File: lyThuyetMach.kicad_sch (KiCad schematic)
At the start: 13 parts, among them J1 USB_C_Receptacle_PowerOnly_6P, J2 Voltage_Booster, J3 TIP223, J4 Out_LED, J5 Clap_Detect, SW1 SW_SPDT, SW2 SW_SPDT, U1 74HC86

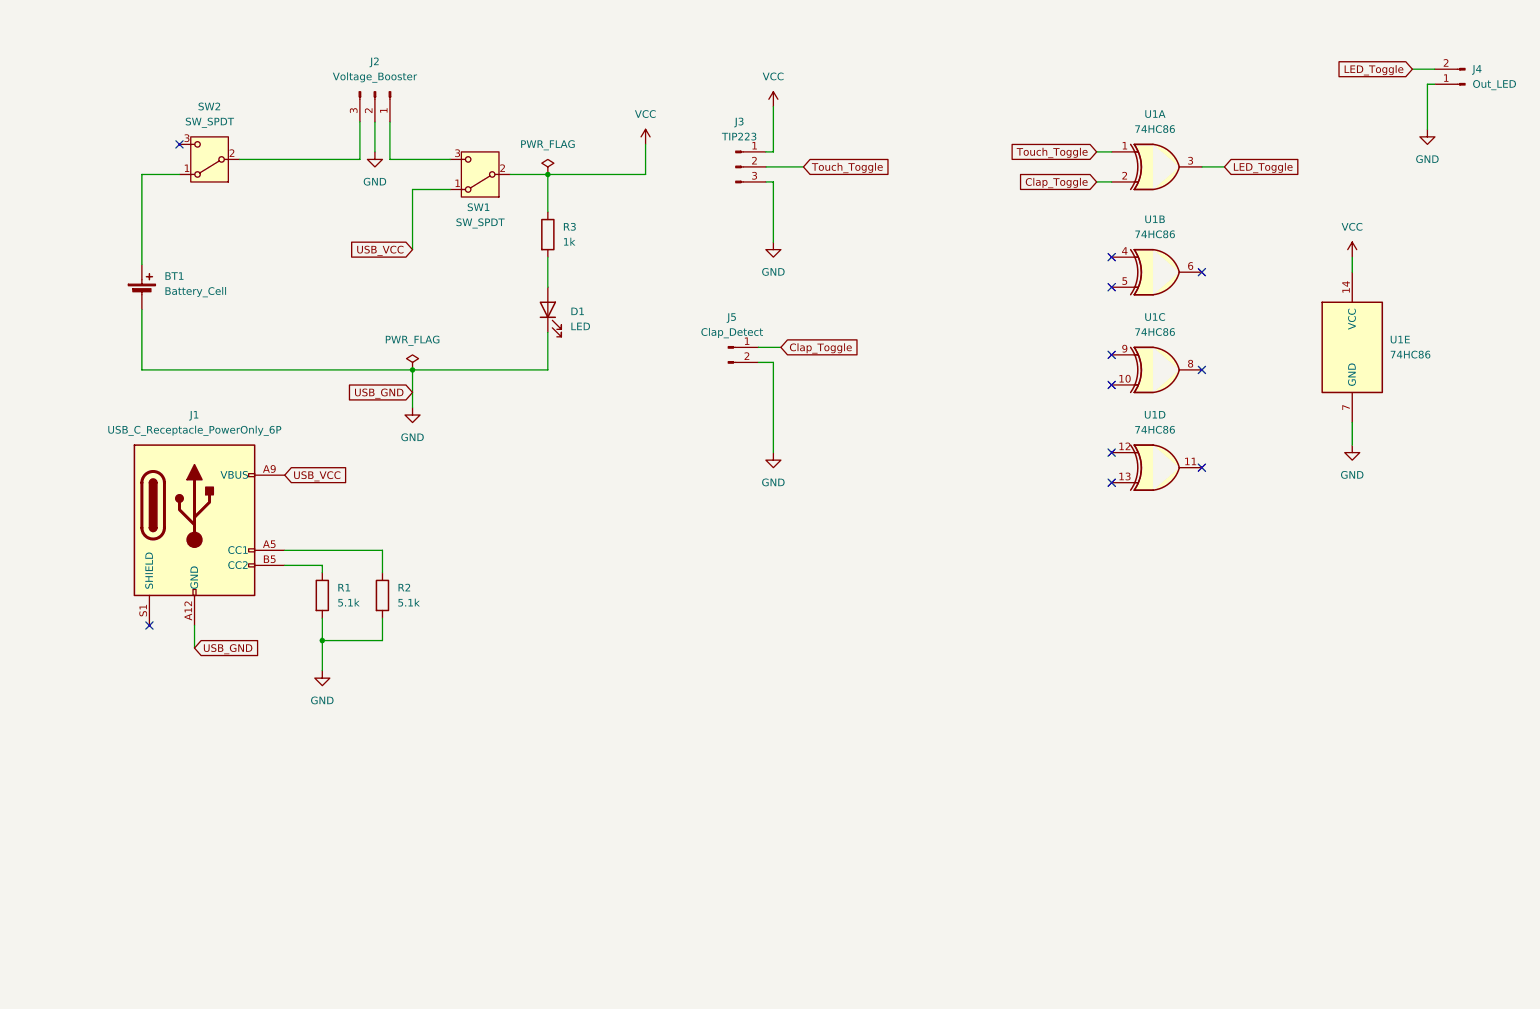
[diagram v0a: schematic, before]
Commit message: Add files via upload
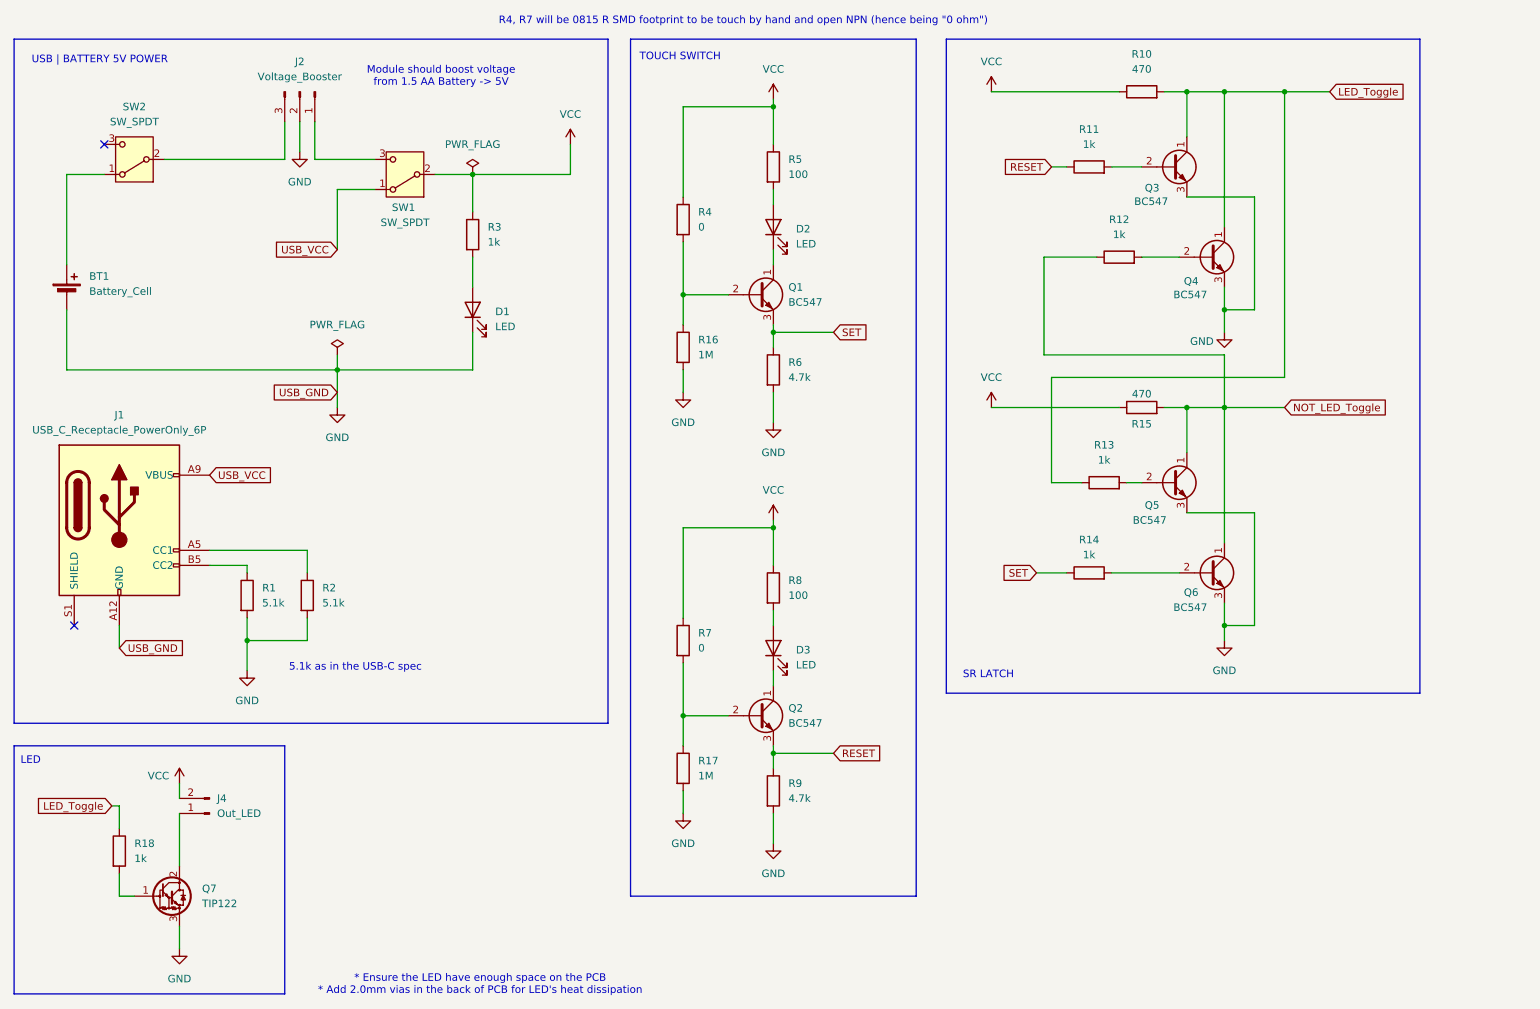
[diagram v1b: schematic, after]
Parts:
- removed J3: TIP223, Connector_PinHeader_2.54mm:PinHeader_1x03_P2.54mm_Vertical, symbol Connector:Conn_01x03_Pin
- removed J5: Clap_Detect, Connector_PinHeader_2.54mm:PinHeader_1x02_P2.54mm_Vertical, symbol Connector:Conn_01x02_Pin
- removed U1: 74HC86, Package_DIP:DIP-14_W7.62mm_Socket_LongPads, symbol 74xx:74HC86
- added D2, D3: LED, LED_THT:LED_D5.0mm_FlatTop, symbol Device:LED
- added Q1, Q2, Q3, Q4, Q5, Q6: BC547, Package_TO_SOT_THT:TO-92_Inline, symbol Transistor_BJT:BC547
- added Q7: TIP122, Package_TO_SOT_THT:TO-220-3_Vertical, symbol Transistor_BJT:TIP122
- added R10, R15: 470, Resistor_THT:R_Axial_DIN0207_L6.3mm_D2.5mm_P10.16mm_Horizontal, symbol Device:R
- added R11, R12, R13, R14, R18: 1k, Resistor_THT:R_Axial_DIN0207_L6.3mm_D2.5mm_P10.16mm_Horizontal, symbol Device:R
- added R16, R17: 1M, Resistor_THT:R_Axial_DIN0207_L6.3mm_D2.5mm_P10.16mm_Horizontal, symbol Device:R
- added R4, R7: 0, Resistor_SMD:R_0815_2038Metric_Pad1.20x4.05mm_HandSolder, symbol Device:R
- added R5, R8: 100, Resistor_THT:R_Axial_DIN0207_L6.3mm_D2.5mm_P10.16mm_Horizontal, symbol Device:R
- added R6, R9: 4.7k, Resistor_THT:R_Axial_DIN0207_L6.3mm_D2.5mm_P10.16mm_Horizontal, symbol Device:R
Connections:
- net GND: now also Q3.3 (E), Q4.3 (E), Q5.3 (E), Q6.3 (E), Q7.3 (E), R16.2, R17.2, R6.2, R9.2; no longer J4.1 (Pin_1)
- net LED_Toggle: now also Q3.1 (C), Q4.1 (C), R10.2, R13.1, R18.1; no longer J4.2 (Pin_2)
- net VCC: now also J4.2 (Pin_2), R10.1, R15.1, R4.1, R5.1, R7.1, R8.1
- new net: Q5.2 (B), R13.2
- new net: Q6.2 (B), R14.2
- new net: Q1.2 (B), R16.1, R4.2
- new net: J4.1 (Pin_1), Q7.2 (C)
- new net: D3.1 (K), Q2.1 (C)
- new net: D3.2 (A), R8.2
- new net: D2.1 (K), Q1.1 (C)
- new net: D2.2 (A), R5.2
- new net: Q3.2 (B), R11.2
- new net: Q4.2 (B), R12.2
- new net: Q2.2 (B), R17.1, R7.2
- new net: Q7.1 (B), R18.2
- new net NOT_LED_Toggle: Q5.1 (C), Q6.1 (C), R12.1, R15.2
- new net RESET: Q2.3 (E), R11.1, R9.1
- new net SET: Q1.3 (E), R14.1, R6.1
- no-connect marks 11 -> 2
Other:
- note added: "* Ensure the LED have enough space on the PCB * Add 2.0mm vias in the back of PCB for LED's heat dissipation"
- note added: "5.1k as in the USB-C spec"
- note added: "LED"
- note added: "Module should boost voltage from 1.5 AA Battery -> 5V"
- note added: "R4, R7 will be 0815 R SMD footprint to be touch by hand and open NPN (hence being "0 ohm")"
- note added: "SR LATCH"
- note added: "TOUCH SWITCH"
- note added: "USB | BATTERY 5V POWER"
- moved on the sheet: BT1, D1, J1, J2, J4, R1, R2, R3, SW1, SW2

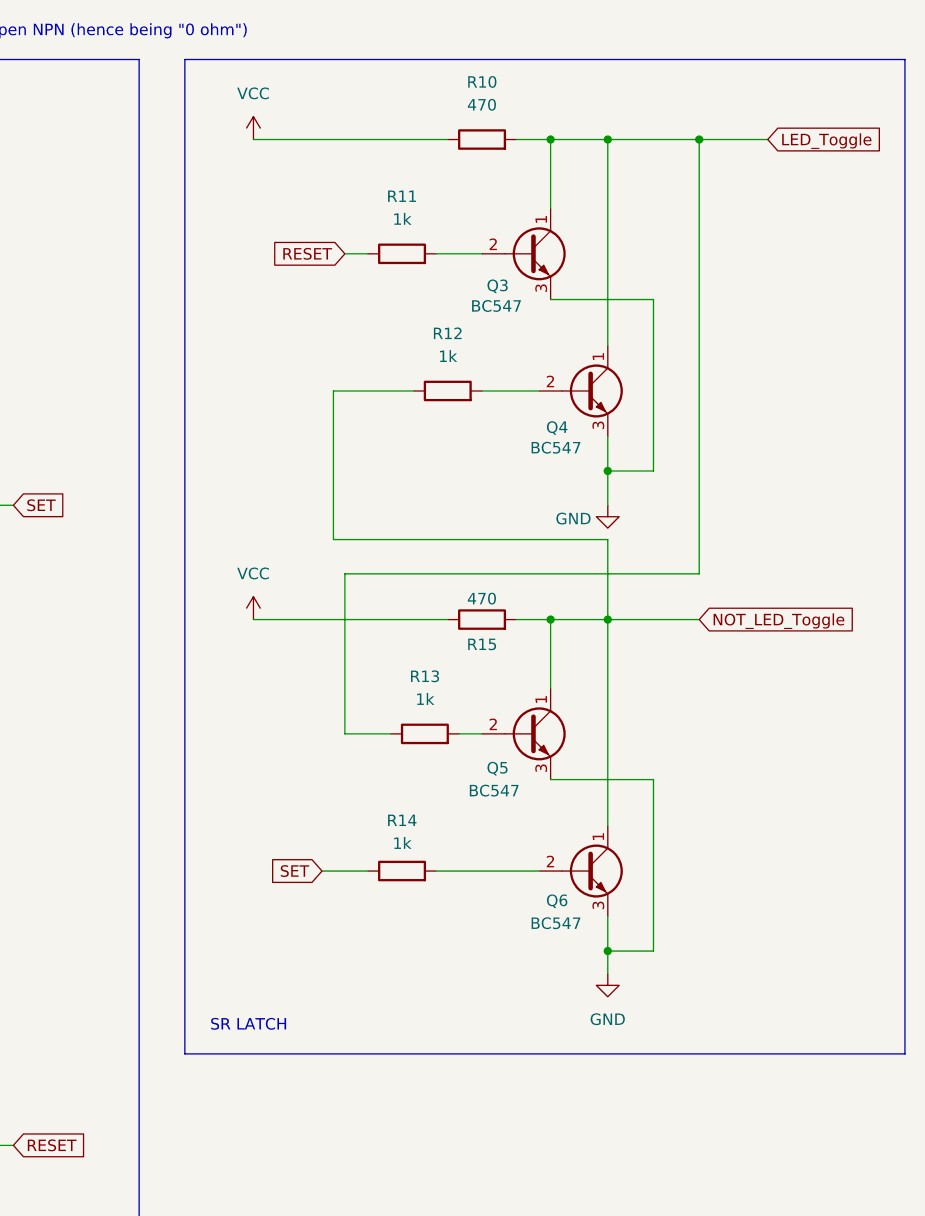
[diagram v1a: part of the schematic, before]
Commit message: Add files via upload
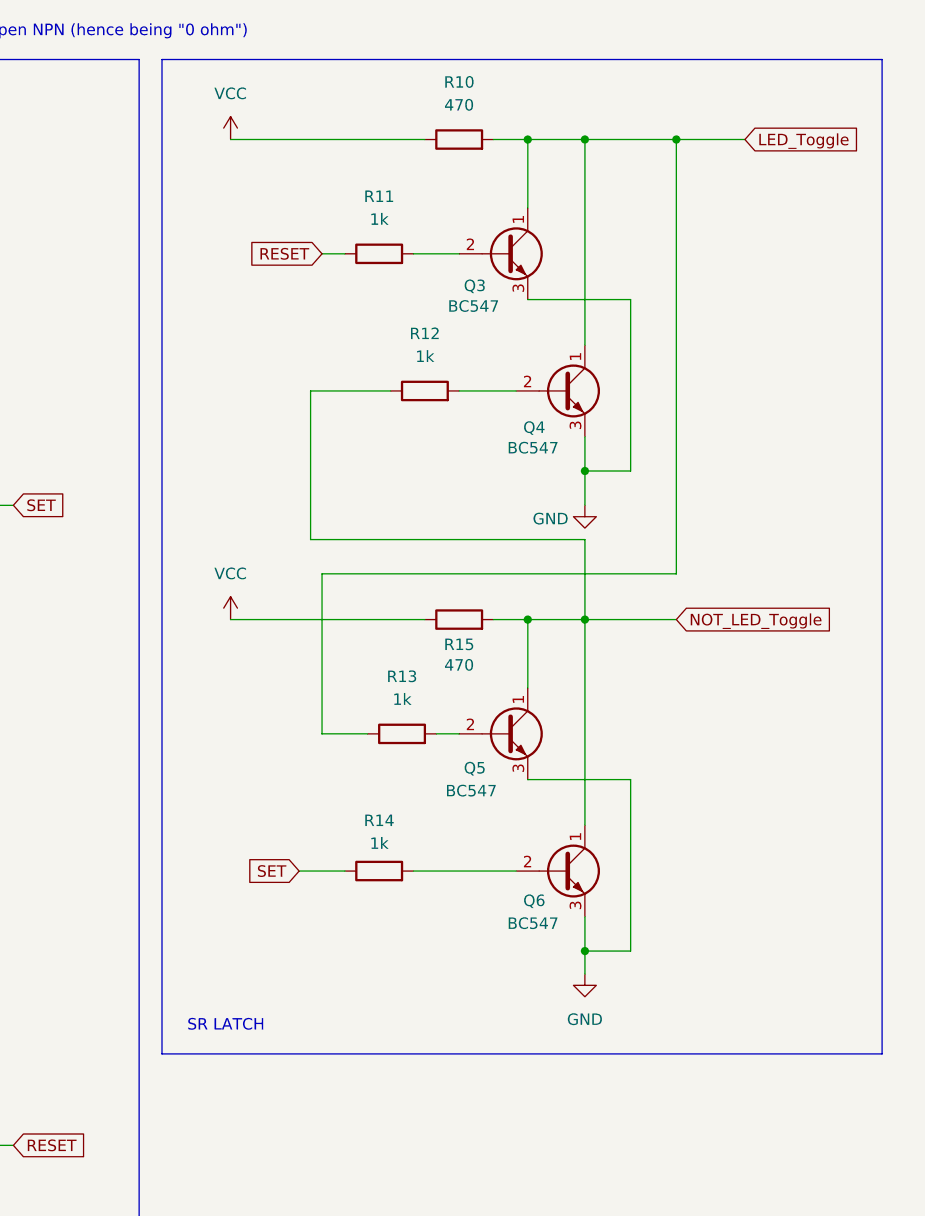
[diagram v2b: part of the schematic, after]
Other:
- moved on the sheet: Q3, Q4, Q5, Q6, R10, R11, R12, R13, R14, R15

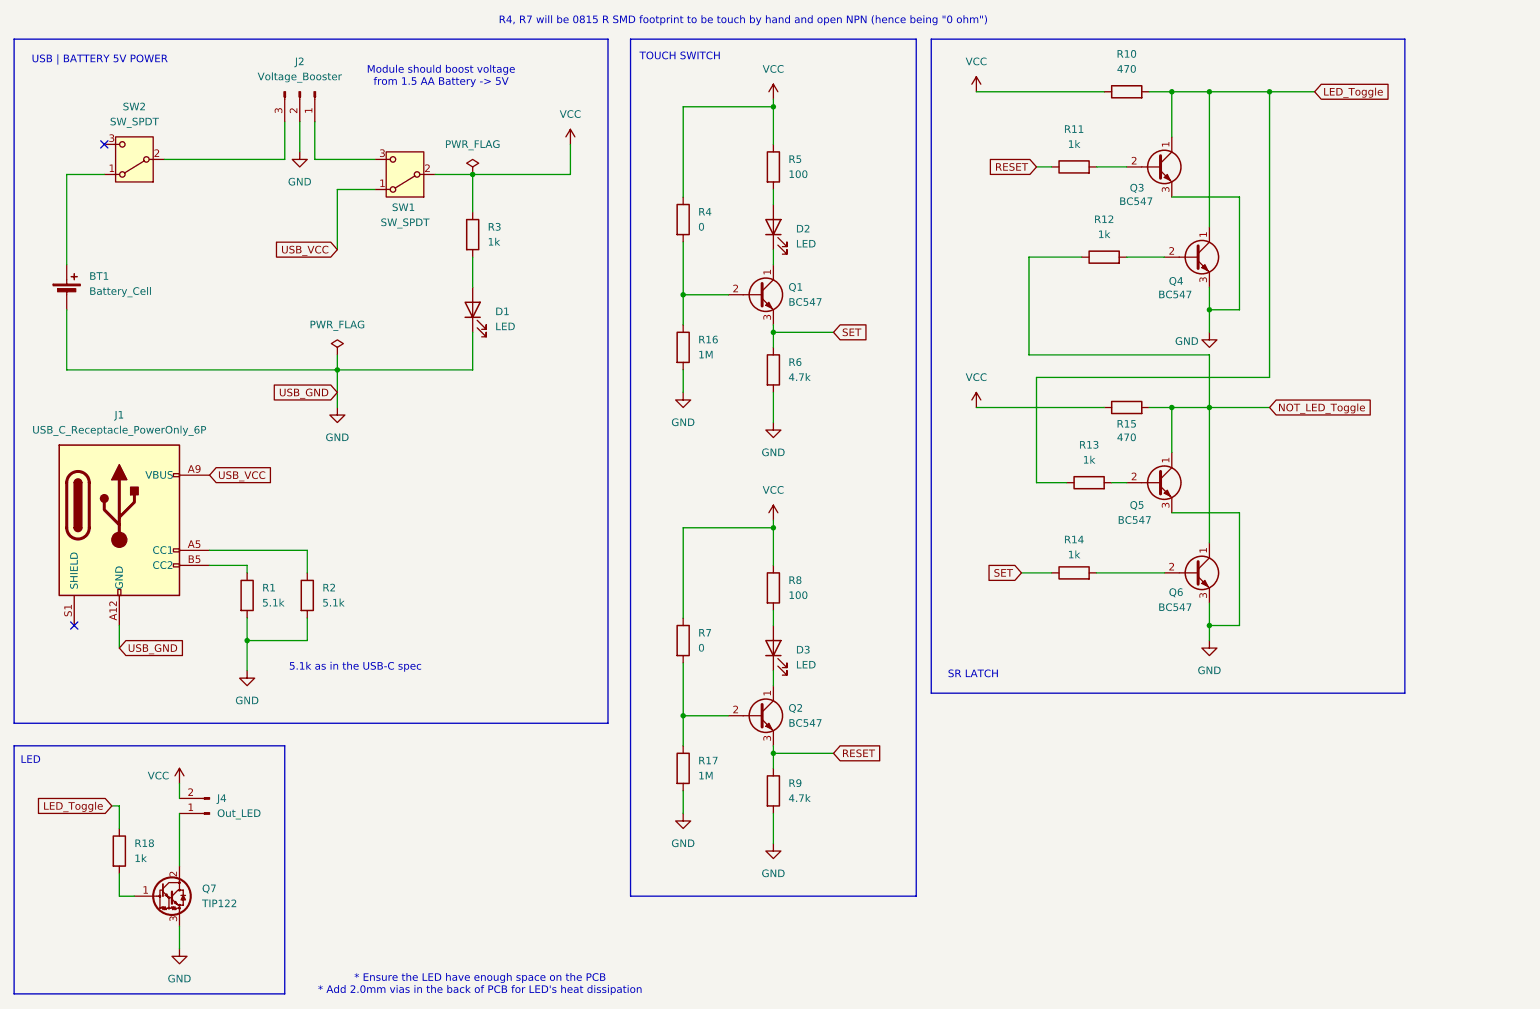
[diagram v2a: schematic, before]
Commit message: Add files via upload
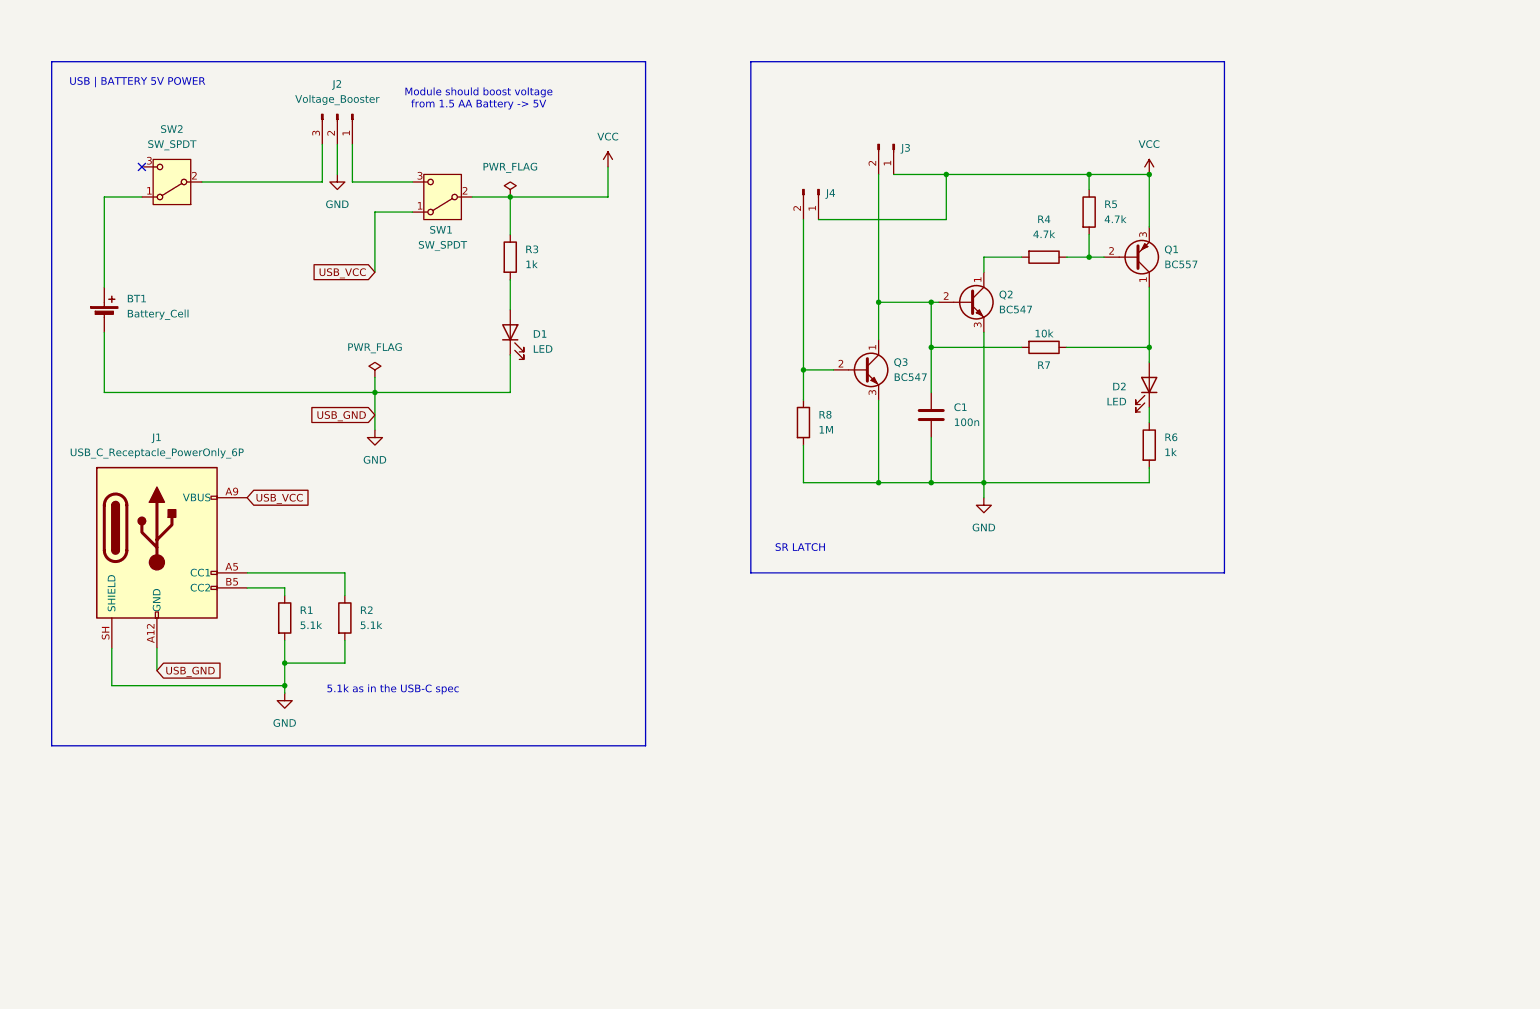
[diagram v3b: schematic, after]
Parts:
- removed D3: LED, LED_THT:LED_D5.0mm_FlatTop, symbol Device:LED
- removed Q1, Q4, Q5, Q6: BC547, Package_TO_SOT_THT:TO-92_Inline, symbol Transistor_BJT:BC547
- removed Q7: TIP122, Package_TO_SOT_THT:TO-220-3_Vertical, symbol Transistor_BJT:TIP122
- removed R10, R15: 470, Resistor_THT:R_Axial_DIN0207_L6.3mm_D2.5mm_P10.16mm_Horizontal, symbol Device:R
- removed R11, R12, R13, R14, R18: 1k, Resistor_THT:R_Axial_DIN0207_L6.3mm_D2.5mm_P10.16mm_Horizontal, symbol Device:R
- removed R16, R17: 1M, Resistor_THT:R_Axial_DIN0207_L6.3mm_D2.5mm_P10.16mm_Horizontal, symbol Device:R
- removed R9: 4.7k, Resistor_THT:R_Axial_DIN0207_L6.3mm_D2.5mm_P10.16mm_Horizontal, symbol Device:R
- added C1: 100n, Capacitor_THT:C_Disc_D5.0mm_W2.5mm_P5.00mm, symbol Device:C
- added J3: Conn_01x02_Pin, Connector_PinHeader_2.54mm:PinHeader_1x02_P2.54mm_Vertical, symbol Connector:Conn_01x02_Pin
- added Q1: BC557, Package_TO_SOT_THT:TO-92_Inline, symbol Transistor_BJT:BC557
- D2: footprint LED_THT:LED_D5.0mm_FlatTop -> LED_THT:LED_D5.0mm
- J4: value Out_LED -> Conn_01x02_Pin
- R4: value 0 -> 4.7k; footprint Resistor_SMD:R_0815_2038Metric_Pad1.20x4.05mm_HandSolder -> Resistor_THT:R_Axial_DIN0207_L6.3mm_D2.5mm_P10.16mm_Horizontal
- R5: value 100 -> 4.7k
- R6: value 4.7k -> 1k
- R7: value 0 -> 10k; footprint Resistor_SMD:R_0815_2038Metric_Pad1.20x4.05mm_HandSolder -> Resistor_THT:R_Axial_DIN0207_L6.3mm_D2.5mm_P10.16mm_Horizontal
- R8: value 100 -> 1M
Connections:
- net LED_Toggle is gone; now on an unnamed net: Q3.1 (C)
- net RESET is gone; now on net GND: Q2.3 (E)
- net SET is gone; now on an unnamed net: R6.1
- net GND: now also J1.SH (SHIELD), R8.2, C1.2
- net VCC: now also J4.1 (Pin_1), J3.1 (Pin_1), Q1.3 (E); no longer J4.2 (Pin_2), R4.1, R7.1, R8.1
- net at R4.2: now also Q2.1 (C)
- net at R5.2: now also R4.1, Q1.2 (B); no longer D2.2 (A)
- net at Q3.2 (B): now also J4.2 (Pin_2), R8.1
- net at Q2.2 (B), R7.2: now also C1.1, J3.2 (Pin_2)
- new net: D2.2 (A), Q1.1 (C), R7.1
- no-connect marks 2 -> 1
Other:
- note removed: "* Ensure the LED have enough space on the PCB * Add 2.0mm vias in the back of PCB for LED's heat dissipation"
- note removed: "LED"
- note removed: "R4, R7 will be 0815 R SMD footprint to be touch by hand and open NPN (hence being "0 ohm")"
- note removed: "TOUCH SWITCH"
- moved on the sheet: BT1, D1, J1, J2, R1, R2, R3, SW1, SW2
